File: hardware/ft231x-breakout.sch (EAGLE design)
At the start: 27 parts, among them Q1 2N7002PW, U1 FT231XS

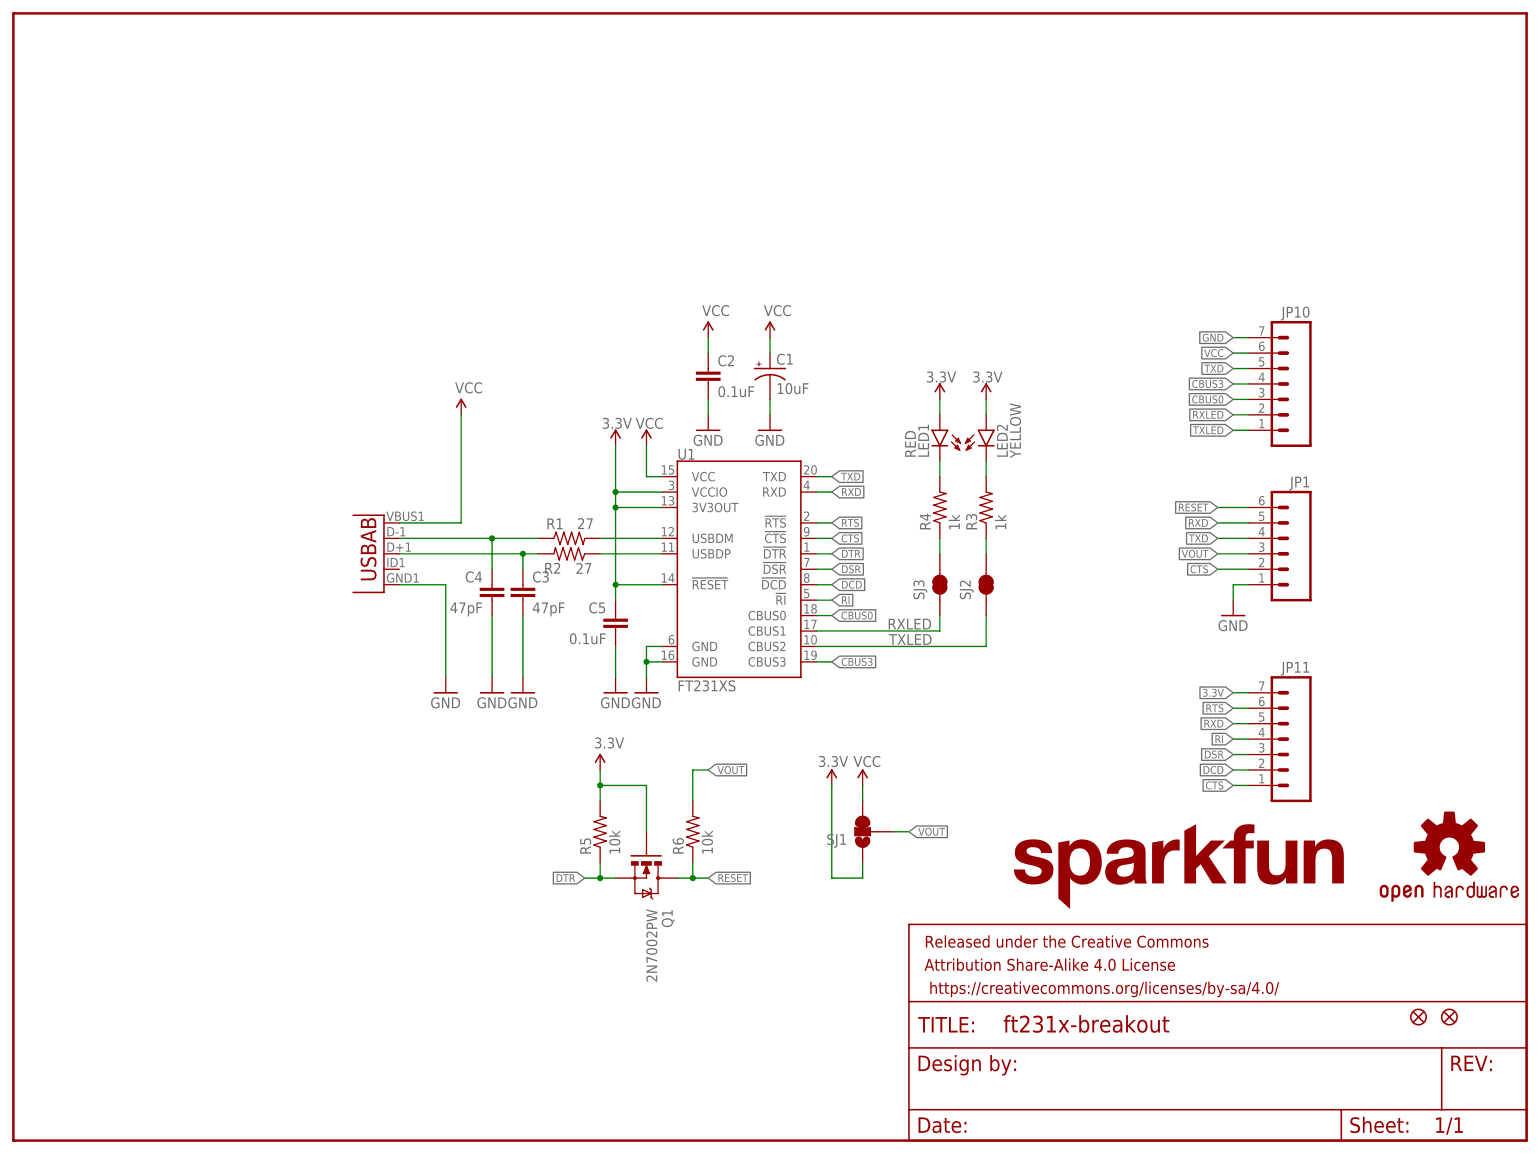
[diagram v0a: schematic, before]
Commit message: Initial QC CL, Updated Parts, Fixed SCH.
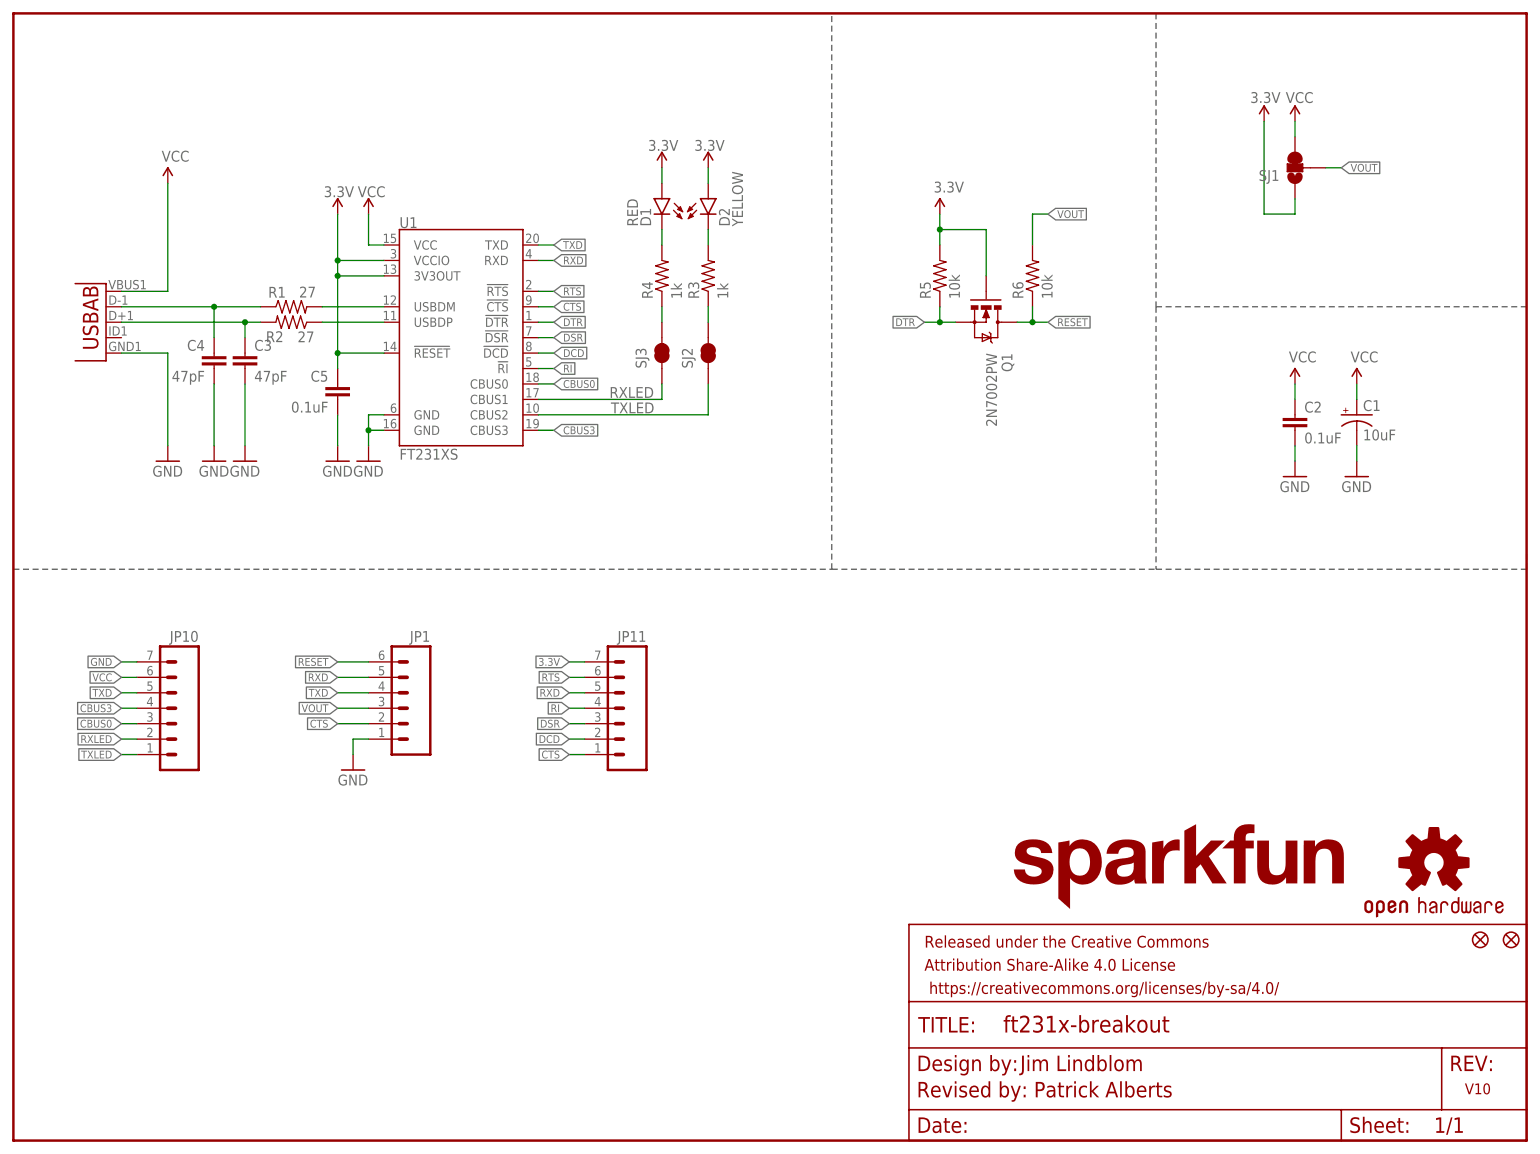
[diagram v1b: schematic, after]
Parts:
- removed LED1: RED, SparkFun-LED:LED0603
- removed LED2: YELLOW, SparkFun-LED:LED-YELLOW0603
- added D1: RED, SparkFun-LED:LED-RED0603
- added D2: YELLOW, SparkFun-LED:LED-YELLOW0603
- C1: device SparkFun-Passives:CAP_POL1206 -> SparkFun-Capacitors:10UF-16V-10%(TANT)
- Q1: device SparkFun-DiscreteSemi:MOSFET-NCHANNELSOT323 -> SparkFun-DiscreteSemi:MOSFET-NCHANNEL2N7002PW
- R1, R2: device SparkFun-Resistors:RESISTOR0603-RES -> SparkFun-Resistors:27OHM1/10W1%(0603)0603-RES
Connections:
- net 3.3V: now also D1.A, D2.A; no longer LED1.A, LED2.A
- net N$5: now also D2.C; no longer LED2.C
- net N$6: now also D1.C; no longer LED1.C
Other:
- note added: "Jim Lindblom"
- note added: "Revised by: Patrick Alberts"
- note added: "V10"
- moved on the sheet: C1, C2, C3, C4, C5, JP1, JP10, JP11, Q1, R1, R2, R3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
